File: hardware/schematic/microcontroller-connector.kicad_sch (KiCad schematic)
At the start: 5 parts, among them J3 Conn_02x12_Odd_Even

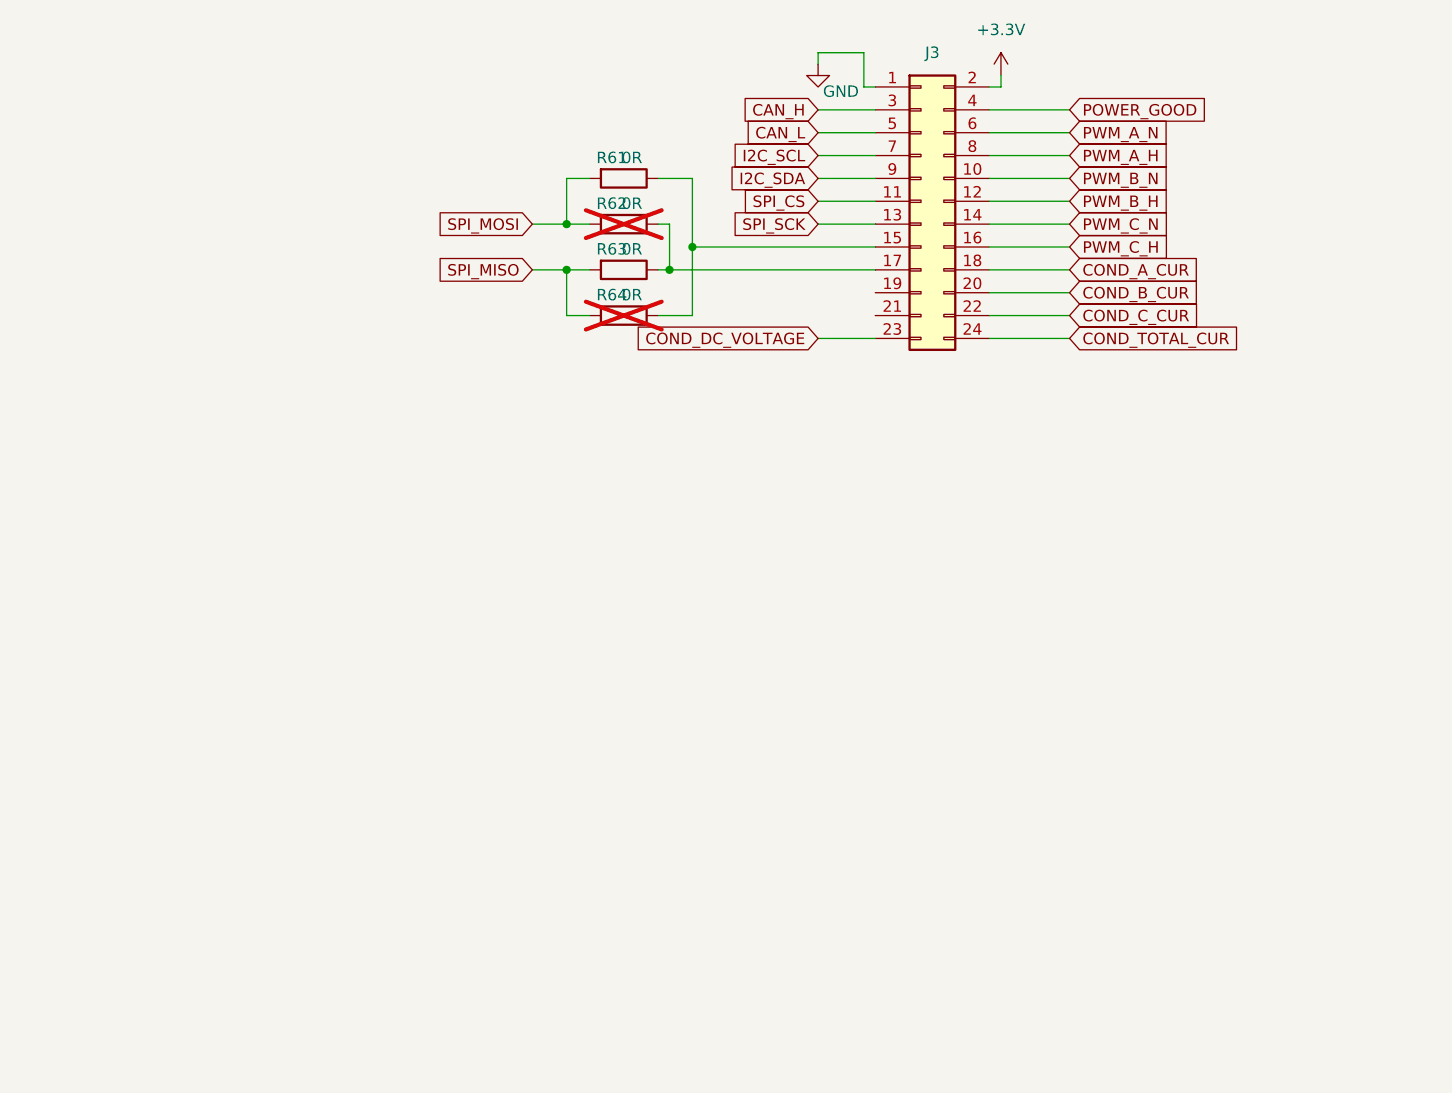
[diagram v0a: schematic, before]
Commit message: schematic finished
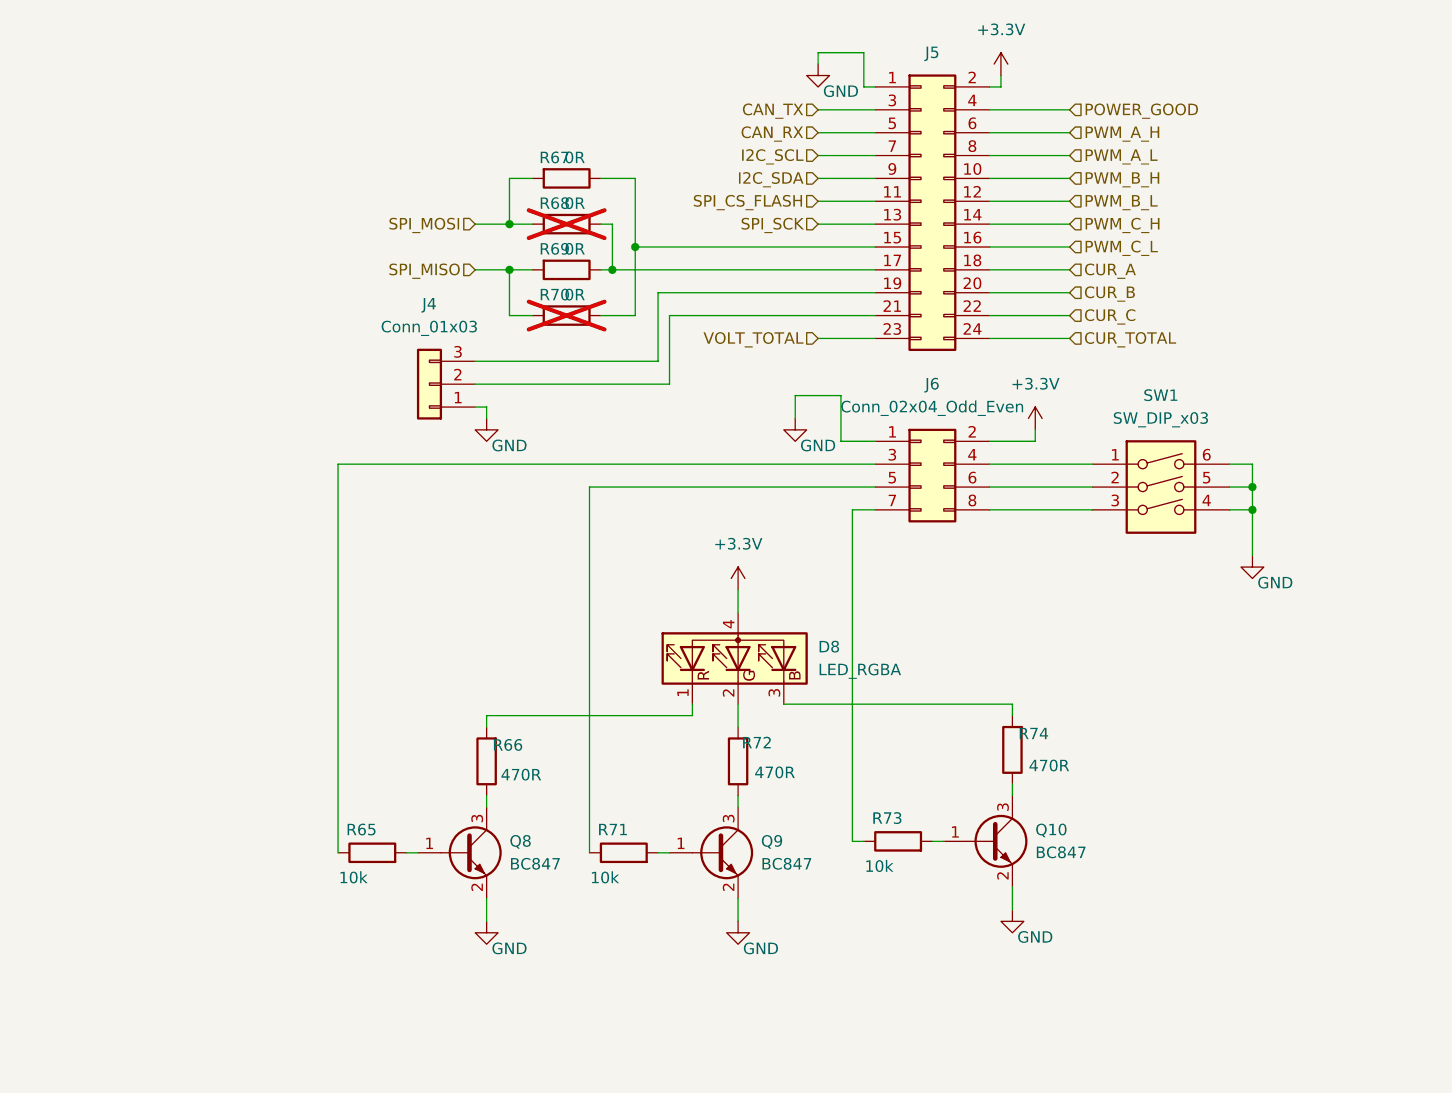
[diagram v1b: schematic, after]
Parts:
- added D8: LED_RGBA, LED_SMD:LED_Cree-PLCC4_5x5mm_CW, symbol Device:LED_RGBA
- added J4: Conn_01x03, Connector_PinSocket_1.27mm:PinSocket_1x03_P1.27mm_Vertical, symbol Connector_Generic:Conn_01x03
- added J6: Conn_02x04_Odd_Even, Connector_PinHeader_1.27mm:PinHeader_2x04_P1.27mm_Horizontal, symbol Connector_Generic:Conn_02x04_Odd_Even
- added Q10, Q8, Q9: BC847, Package_TO_SOT_SMD:SOT-23W_Handsoldering, symbol Transistor_BJT:BC847
- added R65, R71, R73: 10k, Resistor_SMD:R_0805_2012Metric_Pad1.20x1.40mm_HandSolder, symbol Device:R
- added R66, R72, R74: 470R, Resistor_SMD:R_0805_2012Metric_Pad1.20x1.40mm_HandSolder, symbol Device:R
- added SW1: SW_DIP_x03, Button_Switch_SMD:SW_DIP_SPSTx03_Slide_6.7x9.18mm_W8.61mm_P2.54mm_LowProfile, symbol Switch:SW_DIP_x03
- renumbered J3 to J5, R61 to R67, R62 to R68, R63 to R69, R64 to R70
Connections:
- net PWM_A_N is gone; now on net PWM_A_H: J5.6 (Pin_6)
- net PWM_B_N is gone; now on net PWM_B_H: J5.10 (Pin_10)
- net PWM_C_N is gone; now on net PWM_C_H: J5.14 (Pin_14)
- net +3.3V: now also D8.4 (A), J6.2 (Pin_2)
- net GND: now also J4.1 (Pin_1), J6.1 (Pin_1), Q10.2 (E), Q8.2 (E), Q9.2 (E), SW1.4, SW1.5, SW1.6
- net PWM_A_H: no longer J5.8 (Pin_8)
- net PWM_B_H: no longer J5.12 (Pin_12)
- net PWM_C_H: no longer J5.16 (Pin_16)
- net at J5.19 (Pin_19): now also J4.3 (Pin_3)
- net at J5.21 (Pin_21): now also J4.2 (Pin_2)
- net CAN_H renamed CAN_TX
- net CAN_L renamed CAN_RX
- net COND_A_CUR renamed CUR_A
- net COND_B_CUR renamed CUR_B
- net COND_C_CUR renamed CUR_C
- net COND_DC_VOLTAGE renamed VOLT_TOTAL
- net COND_TOTAL_CUR renamed CUR_TOTAL
- net SPI_CS renamed SPI_CS_FLASH
- new net: D8.1 (RK), R66.2
- new net: D8.2 (GK), R72.2
- new net: D8.3 (BK), R74.2
- new net: Q9.3 (C), R72.1
- new net: J6.3 (Pin_3), R65.1
- new net: Q8.1 (B), R65.2
- new net: Q10.3 (C), R74.1
- new net: J6.4 (Pin_4), SW1.1
- new net: J6.6 (Pin_6), SW1.2
- new net: J6.8 (Pin_8), SW1.3
- new net: J6.7 (Pin_7), R73.1
- new net: Q10.1 (B), R73.2
- new net: Q9.1 (B), R71.2
- new net: J6.5 (Pin_5), R71.1
- new net: Q8.3 (C), R66.1
- new net PWM_A_L: J5.8 (Pin_8)
- new net PWM_B_L: J5.12 (Pin_12)
- new net PWM_C_L: J5.16 (Pin_16)
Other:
- moved on the sheet: R67, R68, R69, R70

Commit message: pcb improvements
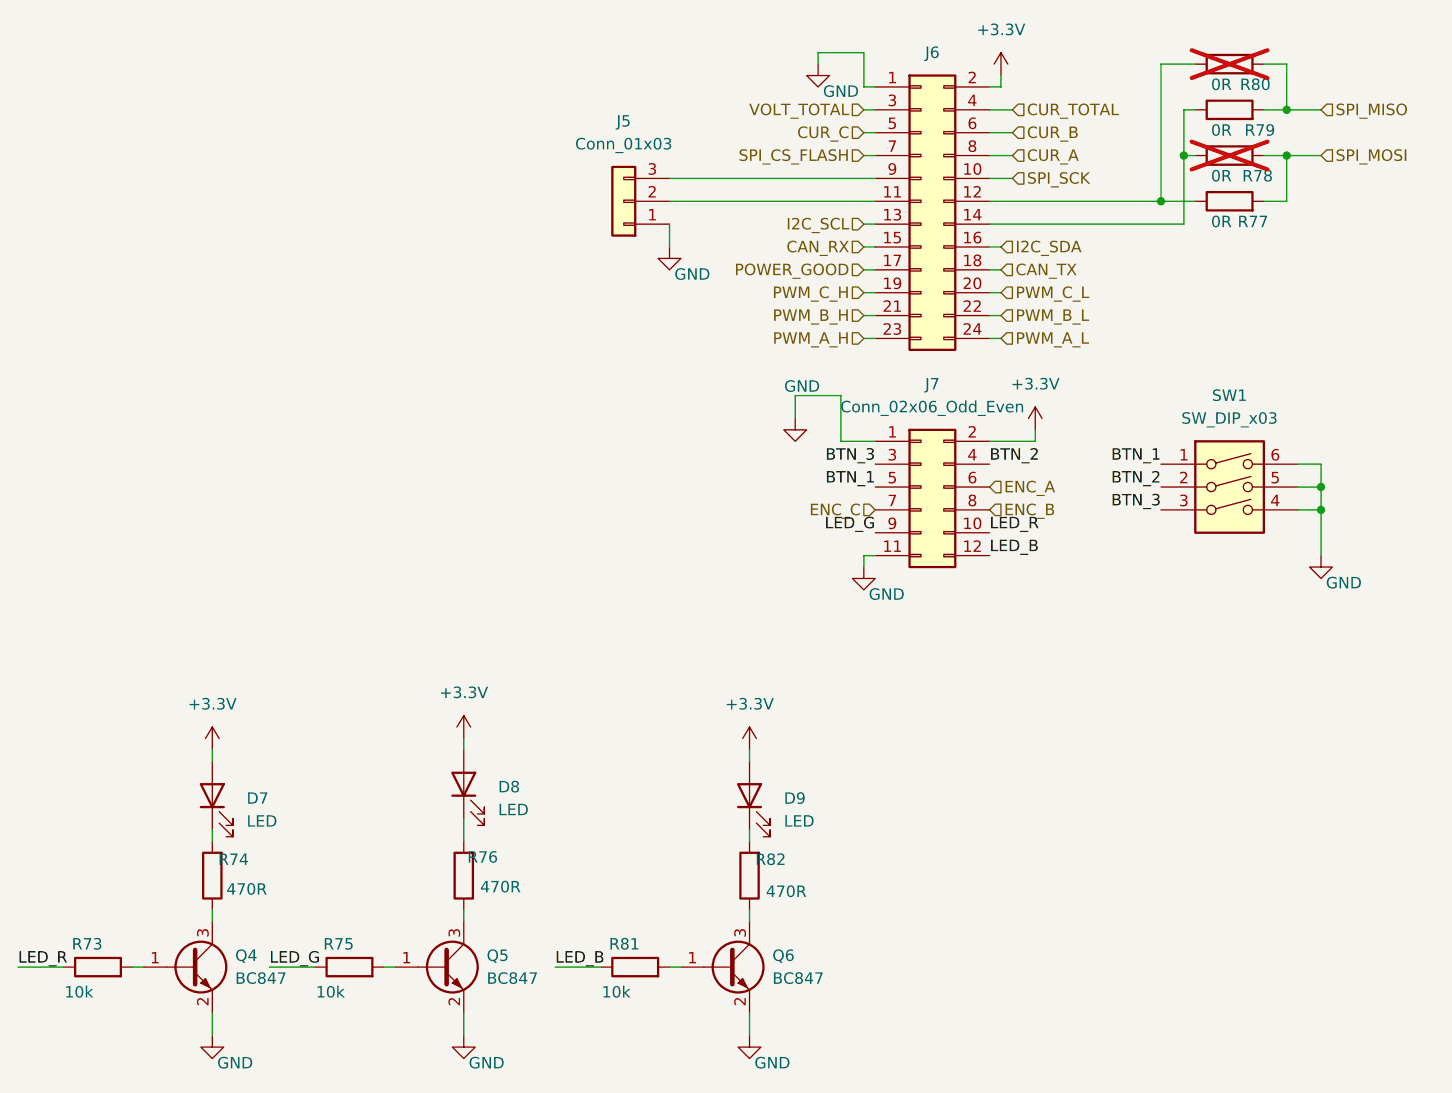
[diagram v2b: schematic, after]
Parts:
- removed D8: LED_RGBA, LED_SMD:LED_Cree-PLCC4_5x5mm_CW, symbol Device:LED_RGBA
- removed J6: Conn_02x04_Odd_Even, Connector_PinHeader_1.27mm:PinHeader_2x04_P1.27mm_Horizontal, symbol Connector_Generic:Conn_02x04_Odd_Even
- added D7, D8, D9: LED, LED_SMD:LED_0805_2012Metric_Pad1.15x1.40mm_HandSolder, symbol Device:LED
- added J7: Conn_02x06_Odd_Even, Connector_PinHeader_2.54mm:PinHeader_2x06_P2.54mm_Vertical, symbol Connector_Generic:Conn_02x06_Odd_Even
- J5: renamed from J4; footprint Connector_PinSocket_1.27mm:PinSocket_1x03_P1.27mm_Vertical -> Connector_PinHeader_2.54mm:PinHeader_1x03_P2.54mm_Vertical
- J6: renamed from J5; footprint Connector_PinHeader_1.27mm:PinHeader_2x12_P1.27mm_Horizontal -> Connector_PinHeader_2.54mm:PinHeader_2x12_P2.54mm_Vertical
- renumbered Q8 to Q4, Q9 to Q5, Q10 to Q6, R65 to R73, R66 to R74, R71 to R75, R72 to R76, R67 to R77, R68 to R78, R69 to R79, R70 to R80, R73 to R81, R74 to R82
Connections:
- net +3.3V: now also D7.2 (A), D8.2 (A), D9.2 (A), J7.2 (Pin_2)
- net CAN_RX: now also J6.15 (Pin_15); no longer J6.5 (Pin_5)
- net CAN_TX: now also J6.18 (Pin_18); no longer J6.3 (Pin_3)
- net CUR_A: now also J6.8 (Pin_8); no longer J6.18 (Pin_18)
- net CUR_B: now also J6.6 (Pin_6); no longer J6.20 (Pin_20)
- net CUR_C: now also J6.5 (Pin_5); no longer J6.22 (Pin_22)
- net CUR_TOTAL: now also J6.4 (Pin_4); no longer J6.24 (Pin_24)
- net GND: now also J7.1 (Pin_1), J7.11 (Pin_11)
- net I2C_SCL: now also J6.13 (Pin_13); no longer J6.7 (Pin_7)
- net I2C_SDA: now also J6.16 (Pin_16); no longer J6.9 (Pin_9)
- net POWER_GOOD: now also J6.17 (Pin_17); no longer J6.4 (Pin_4)
- net PWM_A_H: now also J6.23 (Pin_23); no longer J6.6 (Pin_6)
- net PWM_A_L: now also J6.24 (Pin_24); no longer J6.8 (Pin_8)
- net PWM_B_H: now also J6.21 (Pin_21); no longer J6.10 (Pin_10)
- net PWM_B_L: now also J6.22 (Pin_22); no longer J6.12 (Pin_12)
- net PWM_C_H: now also J6.19 (Pin_19); no longer J6.14 (Pin_14)
- net PWM_C_L: now also J6.20 (Pin_20); no longer J6.16 (Pin_16)
- net SPI_CS_FLASH: now also J6.7 (Pin_7); no longer J6.11 (Pin_11)
- net SPI_SCK: now also J6.10 (Pin_10); no longer J6.13 (Pin_13)
- net VOLT_TOTAL: now also J6.3 (Pin_3); no longer J6.23 (Pin_23)
- net at R74.2: now also D7.1 (K)
- net at R76.2: now also D8.1 (K)
- net at R82.2: now also D9.1 (K)
- net at R78.1, R79.1: now also J6.14 (Pin_14); no longer J6.17 (Pin_17)
- net LED_R: now reaches R73.1
- net LED_R: now also J7.10 (Pin_10)
- net BTN_1: now reaches SW1.1
- net BTN_1: now also J7.5 (Pin_5)
- net BTN_2: now reaches SW1.2
- net BTN_2: now also J7.4 (Pin_4)
- net BTN_3: now reaches SW1.3
- net BTN_3: now also J7.3 (Pin_3)
- net at R77.1, R80.1: now also J6.12 (Pin_12); no longer J6.15 (Pin_15)
- net LED_B: now reaches R81.1
- net LED_B: now also J7.12 (Pin_12)
- net at J5.3 (Pin_3): now also J6.9 (Pin_9); no longer J6.19 (Pin_19)
- net at J5.2 (Pin_2): now also J6.11 (Pin_11); no longer J6.21 (Pin_21)
- net LED_G: now reaches R75.1
- net LED_G: now also J7.9 (Pin_9)
- new net ENC_A: J7.6 (Pin_6)
- new net ENC_B: J7.8 (Pin_8)
- new net ENC_C: J7.7 (Pin_7)
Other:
- moved on the sheet: J5, Q4, Q5, Q6, R73, R74, R75, R76, R77, R78, R79, R80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
